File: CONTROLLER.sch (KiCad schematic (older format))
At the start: 74 parts, among them J23 Conn_02x03_Odd_Even, J24 ICSP, J25 Raspberry_Pi_2_3, Q13 DTC124E, Q14 DTC124E, Q15 DTC124E, Q16 DTC124E, Q17 DTC124E, Q18 BCX53, U11 CD4052B, U12 74LVC2G14, U13 74LVC2G14, U14 ATmega8-16AU, U15 SN74LVC1G11DBVR, U16 SN74LVC1G11DBVR, U17 MCP23017_SO, U18 MAX11616, U19 TXS0108EPW, U20 TXS0108EPW, U21 TXS0108EPW, U22 MCP23017_SO, U23 MAX3232

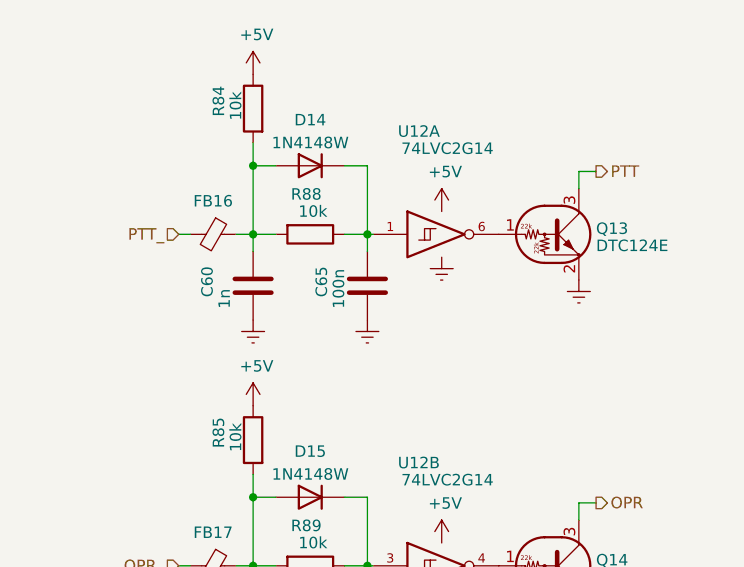
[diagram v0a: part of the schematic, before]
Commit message: RC1
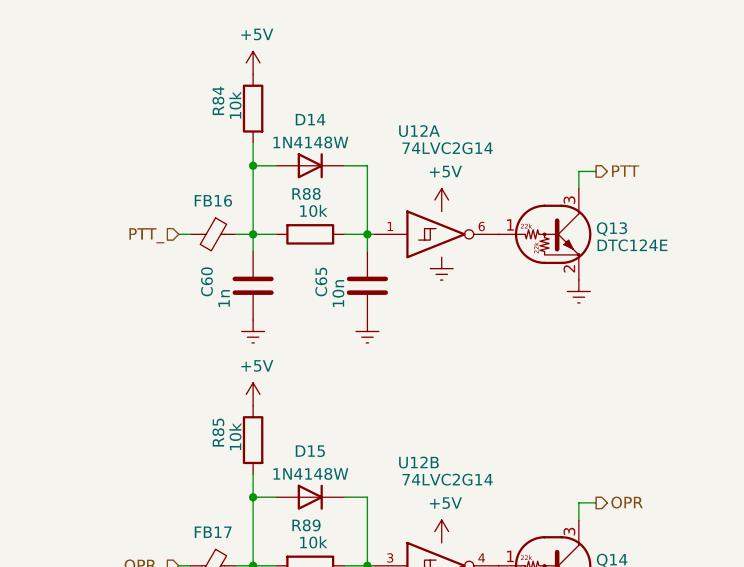
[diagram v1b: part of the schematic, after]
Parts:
- C65: value 100n -> 10n
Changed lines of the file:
@@
 AR Path="/5CBD59C6/5FB02049" Ref="C65"  Part="1"
 F 0 "C65" V 2400 6425 50  0000 L CNN
-F 1 "100n" V 2325 6375 50  0000 L CNN
+F 1 "10n" V 2325 6375 50  0000 L CNN
 F 2 "Capacitor_SMD:C_0805_2012Metric_Pad1.15x1.40mm_HandSolder" H 2238 6325 50  0001 C CNN
 F 3 "~" H 2200 6475 50  0001 C CNN
